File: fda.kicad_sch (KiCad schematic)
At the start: 43 parts, among them U706 OPA2197D, U73 OPA2388DGK, U74 THS4521IDGK

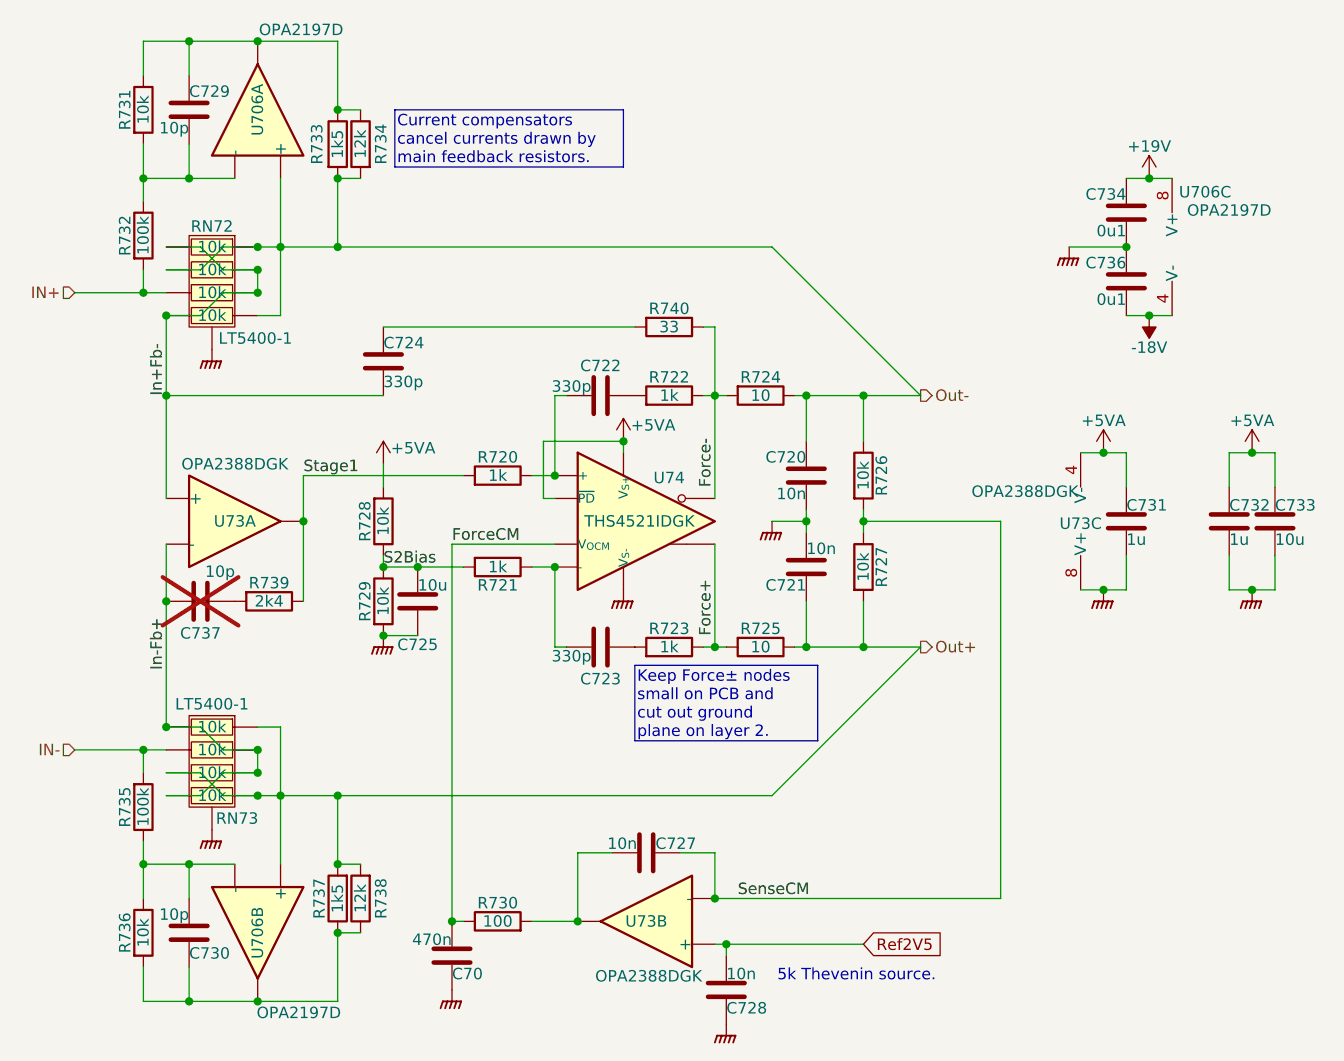
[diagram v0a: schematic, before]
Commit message: Progress checkin.  About to redo FDA feedback again.
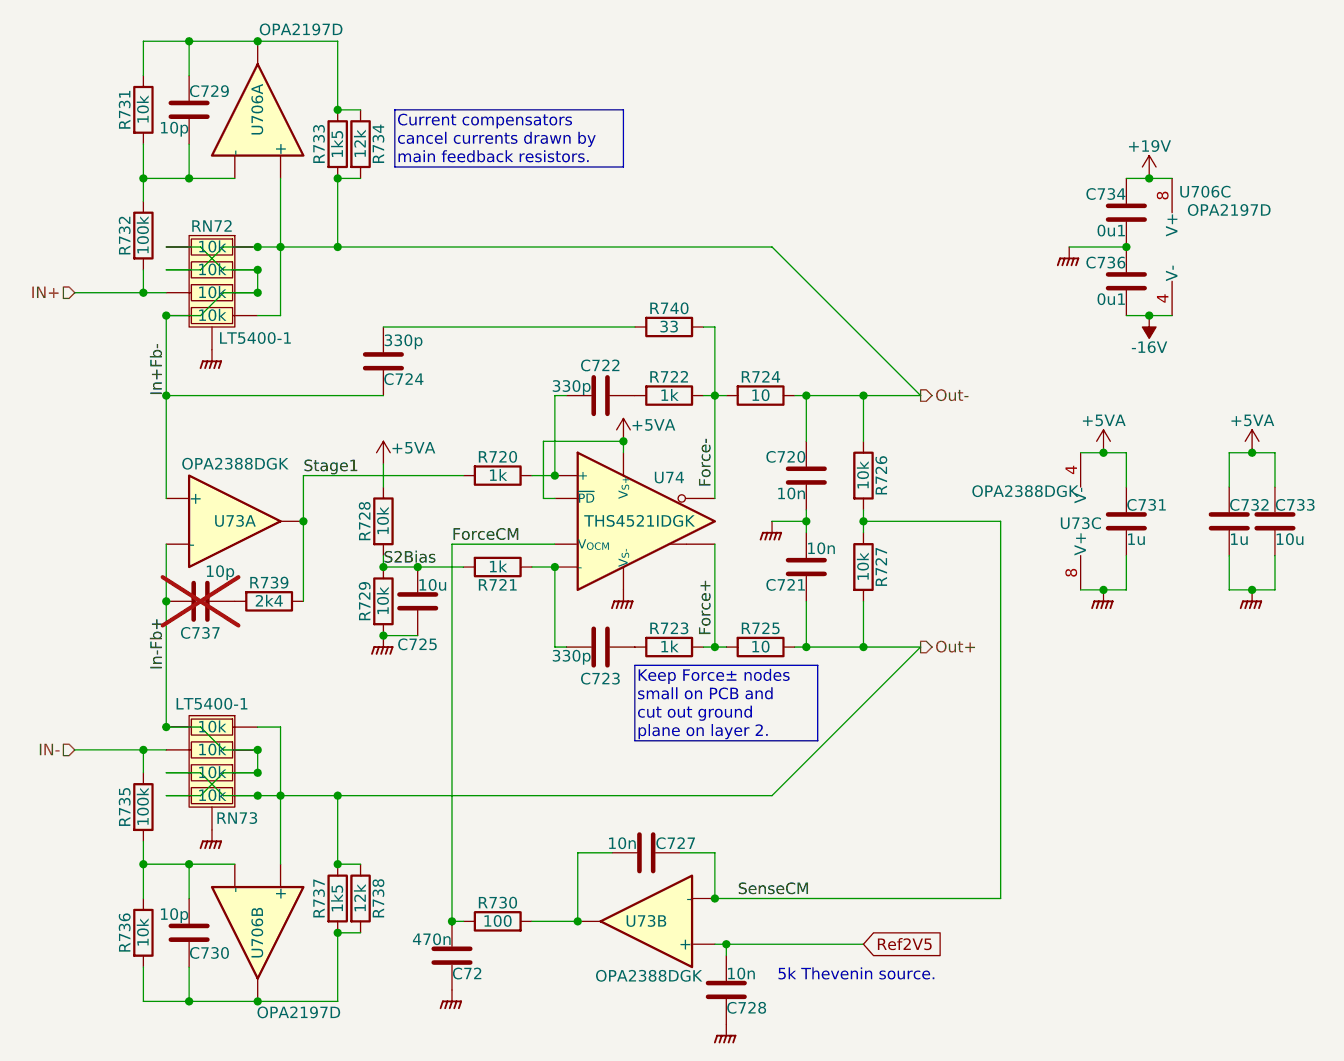
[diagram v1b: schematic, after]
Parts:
- renumbered C70 to C72
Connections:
- net +5VA: now also R728.1; no longer R728.2
- net IN-: now also R735.1; no longer R735.2
- net In+Fb-: now also C724.2; no longer C724.1
- net Out+: now also R737.1, R738.1; no longer R737.2, R738.2
- net S2Bias: now also R728.2; no longer R728.1
- net at C730.2, R736.2, U706.7: now also R737.2, R738.2; no longer R737.1, R738.1
- net at R740.2: now also C724.1; no longer C724.2
- net at C730.1, R736.1, U706.6 (-): now also R735.2; no longer R735.1
- net -18V renamed -16V
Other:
- moved on the sheet: C724, R737, R738
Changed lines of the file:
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@@
 		(lib_id "Device:R")
 		(at 128.27 118.11 270)
-		(mirror x)
 		(unit 1)
 		(exclude_from_sim no)
@@
 		)
 		(property "Footprint" "Resistor_SMD:R_0402_1005Metric"
-			(at 128.27 119.888 90)
+			(at 128.27 116.332 90)
 			(effects
 				(font
@@
 		(lib_id "Device:R")
 		(at 128.27 90.17 270)
-		(mirror x)
 		(unit 1)
 		(exclude_from_sim no)
@@
 		)
 		(property "Footprint" "Resistor_SMD:R_0402_1005Metric"
-			(at 128.27 91.948 90)
+			(at 128.27 88.392 90)
 			(effects
 				(font
@@
 		(lib_id "Device:R")
 		(at 109.22 99.06 270)
-		(mirror x)
 		(unit 1)
 		(exclude_from_sim no)
@@
 		)
 		(property "Footprint" "Resistor_SMD:R_0402_1005Metric"
-			(at 109.22 100.838 90)
+			(at 109.22 97.282 90)
 			(effects
 				(font
@@
 		(lib_id "Device:C")
 		(at 143.51 99.06 0)
-		(mirror y)
 		(unit 1)
 		(exclude_from_sim no)
@@
 					(size 1.27 1.27)
 				)
-				(justify left)
+				(justify right)
 			)
 		)
@@
 					(size 1.27 1.27)
 				)
-				(justify left)
+				(justify right)
 			)
 		)
 		(property "Footprint" "Capacitor_SMD:C_0603_1608Metric"
-			(at 142.5448 102.87 0)
+			(at 144.4752 102.87 0)
 			(effects
 				(font
@@
 		(lib_id "Device:R")
 		(at 96.52 104.14 0)
-		(mirror x)
 		(unit 1)
 		(exclude_from_sim no)
@@
 	(symbol
 		(lib_id "Device:R")
-		(at 91.44 146.05 180)
+		(at 91.44 146.05 0)
 		(unit 1)
 		(exclude_from_sim no)
@@
 		)
 		(property "Footprint" "Resistor_SMD:R_0402_1005Metric"
-			(at 93.218 146.05 90)
+			(at 89.662 146.05 90)
 			(effects
 				(font
@@
 		(on_board yes)
 		(dnp no)
-		(property "Reference" "C70"
+		(property "Reference" "C72"
 			(at 104.14 154.432 0)
 			(effects
@@
 			(project "lincal"
 				(path "/b054cef4-39e3-49d8-aff0-7ba5a206c187/91ba7742-b0d4-4498-bde0-79d5f38f349f"
-					(reference "C70")
+					(reference "C72")
 					(unit 1)
 				)
@@
 	(symbol
 		(lib_id "Device:R")
-		(at 93.98 146.05 180)
+		(at 93.98 146.05 0)
 		(unit 1)
 		(exclude_from_sim no)
@@
 		(dnp no)
 		(property "Reference" "R738"
-			(at 96.266 146.05 90)
+			(at 96.012 146.05 90)
 			(effects
 				(font
@@
 		)
 		(property "Footprint" "Resistor_SMD:R_0603_1608Metric"
-			(at 95.758 146.05 90)
+			(at 92.202 146.05 90)
 			(effects
 				(font
@@
 		(dnp no)
 		(property "Reference" "R733"
-			(at 89.154 62.23 90)
+			(at 89.408 62.23 90)
 			(effects
 				(font
@@
 	(symbol
 		(lib_id "Device:C")
-		(at 96.52 86.36 180)
+		(at 96.52 86.36 0)
 		(unit 1)
 		(exclude_from_sim no)
@@
 		(dnp no)
 		(property "Reference" "C724"
-			(at 96.52 84.328 0)
+			(at 96.52 88.392 0)
 			(effects
 				(font
 					(size 1.27 1.27)
 				)
-				(justify right)
+				(justify left)
 			)
 		)
 		(property "Value" "330p"
-			(at 96.52 88.646 0)
+			(at 96.52 84.074 0)
 			(effects
 				(font
 					(size 1.27 1.27)
 				)
-				(justify right)
+				(justify left)
 			)
 		)
 		(property "Footprint" "Capacitor_SMD:C_0603_1608Metric"
-			(at 95.5548 82.55 0)
+			(at 97.4852 90.17 0)
 			(effects
 				(font
@@
 		(lib_id "Device:R")
 		(at 93.98 62.23 0)
-		(mirror y)
 		(unit 1)
 		(exclude_from_sim no)
@@
 		(dnp no)
 		(property "Reference" "R734"
-			(at 96.266 62.23 90)
+			(at 96.012 62.23 90)
 			(effects
 				(font
@@
 		)
 		(property "Footprint" "Resistor_SMD:R_0603_1608Metric"
-			(at 95.758 62.23 90)
+			(at 92.202 62.23 90)
 			(effects
 				(font
@@
 	)
 	(symbol
-		(lib_id "Parts:-18V")
+		(lib_id "Parts:-16V")
 		(at 181.61 81.28 0)
 		(unit 1)
@@
 		(on_board yes)
 		(dnp no)
-		(property "Reference" "#PWR0149"
+		(property "Reference" "#PWR149"
 			(at 181.61 77.47 0)
 			(effects
@@
 			)
 		)
-		(property "Value" "-18V"
+		(property "Value" "-16V"
 			(at 181.61 84.836 0)
 			(do_not_autoplace yes)
@@
 			)
 		)
-		(property "Description" "Power symbol creates a global label with name \"-18V\""
+		(property "Description" "Power symbol creates a global label with name \"-16V\""
 			(at 181.61 81.28 0)
 			(effects
@@
 			(project "lincal"
 				(path "/b054cef4-39e3-49d8-aff0-7ba5a206c187/91ba7742-b0d4-4498-bde0-79d5f38f349f"
-					(reference "#PWR0149")
+					(reference "#PWR149")
 					(unit 1)
 				)
@@
 		(lib_id "Device:R")
 		(at 69.85 135.89 0)
-		(mirror x)
 		(unit 1)
 		(exclude_from_sim no)
